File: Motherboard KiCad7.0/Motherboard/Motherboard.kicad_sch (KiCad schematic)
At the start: 52 parts, among them J1 USB_B_Micro, J2 SWD_01x04_Pin, J3 2-1445057-2, Q1 AO3400A, Q2 NMOS, SW1 SW_STM_RESET, SW2 SW_STM_BOOT_MODE, U1 STM32F103CBT6, U2 AMS1117-3.3, U3 LM66100DCKR, U4 LM66100DCKR, U5 LM66100DCKR, Y1 X322516MMB4SI

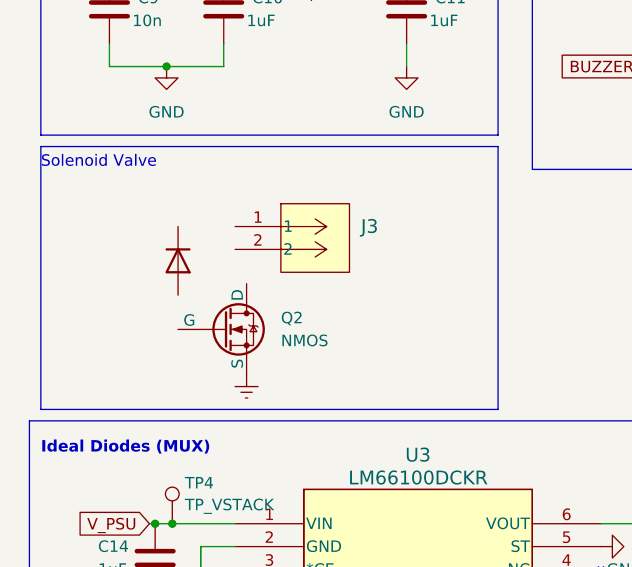
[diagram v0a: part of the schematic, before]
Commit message: Solenoid valve
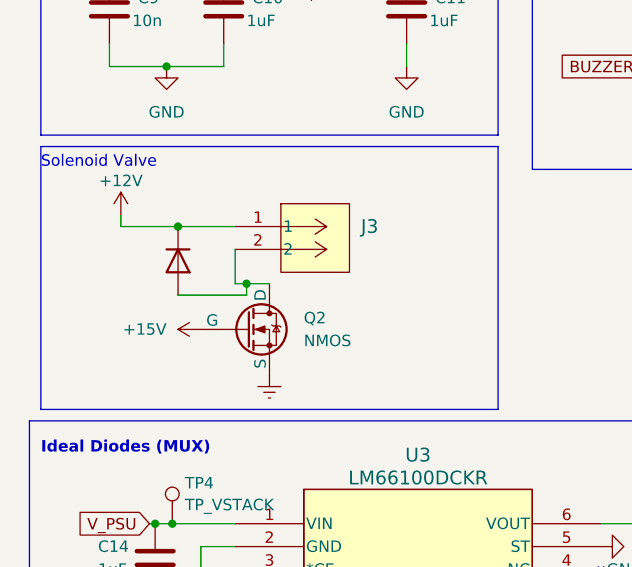
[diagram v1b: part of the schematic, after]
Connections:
- net +12V: now reaches J3.1
- net +12V: now also D6.1 (K)
- net at J3.2: now also D6.2 (A), Q2.1 (D)
- net +15V: now reaches Q2.2 (G)
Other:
- moved on the sheet: Q2
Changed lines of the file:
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@@
   (junction (at 175.26 110.49) (diameter 0) (color 0 0 0 0)
+  )
+  (junction (at 39.37 114.3) (diameter 0) (color 0 0 0 0)
+  )
+  (junction (at 31.75 107.95) (diameter 0) (color 0 0 0 0)
   )
   (junction (at 29.21 186.69) (diameter 0) (color 0 0 0 0)
@@
     (stroke (width 0) (type default))
   )
+  (wire (pts (xy 25.4 106.68) (xy 25.4 107.95))
+    (stroke (width 0) (type default))
+  )
   (wire (pts (xy 116.84 175.26) (xy 119.38 175.26))
     (stroke (width 0) (type default))
@@
     (stroke (width 0) (type default))
   )
+  (wire (pts (xy 39.37 114.3) (xy 41.91 114.3))
+    (stroke (width 0) (type default))
+  )
   (wire (pts (xy 241.935 67.31) (xy 245.11 67.31))
     (stroke (width 0) (type default))
@@
     (stroke (width 0) (type default))
   )
+  (wire (pts (xy 39.37 115.57) (xy 39.37 114.3))
+    (stroke (width 0) (type default))
+  )
   (wire (pts (xy 38.1 181.61) (xy 34.29 181.61))
     (stroke (width 0) (type default))
@@
     (stroke (width 0) (type default))
   )
+  (wire (pts (xy 38.1 107.95) (xy 31.75 107.95))
+    (stroke (width 0) (type default))
+  )
   (wire (pts (xy 101.6 36.83) (xy 111.76 36.83))
     (stroke (width 0) (type default))
@@
     (stroke (width 0) (type default))
   )
+  (wire (pts (xy 31.75 115.57) (xy 39.37 115.57))
+    (stroke (width 0) (type default))
+  )
   (wire (pts (xy 57.15 87.63) (xy 57.15 90.17))
     (stroke (width 0) (type default))
@@
     (stroke (width 0) (type default))
   )
+  (wire (pts (xy 38.1 114.3) (xy 39.37 114.3))
+    (stroke (width 0) (type default))
+  )
   (wire (pts (xy 260.35 88.9) (xy 264.16 88.9))
     (stroke (width 0) (type default))
@@
     (stroke (width 0) (type default))
   )
+  (wire (pts (xy 38.1 110.49) (xy 38.1 114.3))
+    (stroke (width 0) (type default))
+  )
   (wire (pts (xy 91.44 90.17) (xy 91.44 91.44))
     (stroke (width 0) (type default))
@@
   )
   (wire (pts (xy 175.26 29.21) (xy 172.72 29.21))
+    (stroke (width 0) (type default))
+  )
+  (wire (pts (xy 31.75 107.95) (xy 25.4 107.95))
     (stroke (width 0) (type default))
   )
@@
     )
   )
-  (symbol (lib_id "power:Earth") (at 39.37 124.46 0) (unit 1)
-    (in_bom yes) (on_board yes) (dnp no) (fields_autoplaced)
-    (property "Reference" "#PWR033" (at 39.37 130.81 0)
-      (effects (font (size 1.27 1.27)) hide)
-    )
-    (property "Value" "Earth" (at 39.37 128.27 0)
-      (effects (font (size 1.27 1.27)) hide)
-    )
-    (property "Footprint" "" (at 39.37 124.46 0)
-      (effects (font (size 1.27 1.27)) hide)
-    )
-    (property "Datasheet" "~" (at 39.37 124.46 0)
+  (symbol (lib_id "power:Earth") (at 41.91 124.46 0) (unit 1)
+    (in_bom yes) (on_board yes) (dnp no) (fields_autoplaced)
+    (property "Reference" "#PWR033" (at 41.91 130.81 0)
+      (effects (font (size 1.27 1.27)) hide)
+    )
+    (property "Value" "Earth" (at 41.91 128.27 0)
+      (effects (font (size 1.27 1.27)) hide)
+    )
+    (property "Footprint" "" (at 41.91 124.46 0)
+      (effects (font (size 1.27 1.27)) hide)
+    )
+    (property "Datasheet" "~" (at 41.91 124.46 0)
       (effects (font (size 1.27 1.27)) hide)
     )
@@
     )
   )
+  (symbol (lib_id "power:+12V") (at 25.4 106.68 0) (unit 1)
+    (in_bom yes) (on_board yes) (dnp no)
+    (property "Reference" "#PWR034" (at 25.4 110.49 0)
+      (effects (font (size 1.27 1.27)) hide)
+    )
+    (property "Value" "+12V" (at 25.4 102.87 0)
+      (effects (font (size 1.27 1.27)))
+    )
+    (property "Footprint" "" (at 25.4 106.68 0)
+      (effects (font (size 1.27 1.27)) hide)
+    )
+    (property "Datasheet" "" (at 25.4 106.68 0)
+      (effects (font (size 1.27 1.27)) hide)
+    )
+    (pin "1")
+    (instances
+      (project "Motherboard"
+        (path "/6c6aab7b-9fc7-4161-8073-41667e18c629"
+          (reference "#PWR034") (unit 1)
+        )
+      )
+    )
+  )
   (symbol (lib_id "Device:R") (at 228.6 134.62 180) (unit 1)
     (in_bom yes) (on_board yes) (dnp no) (fields_autoplaced)
@@
     )
   )
+  (symbol (lib_id "power:+15V") (at 34.29 119.38 90) (unit 1)
+    (in_bom yes) (on_board yes) (dnp no) (fields_autoplaced)
+    (property "Reference" "#PWR035" (at 38.1 119.38 0)
+      (effects (font (size 1.27 1.27)) hide)
+    )
+    (property "Value" "+15V" (at 30.48 119.38 90)
+      (effects (font (size 1.27 1.27)) (justify left))
+    )
+    (property "Footprint" "" (at 34.29 119.38 0)
+      (effects (font (size 1.27 1.27)) hide)
+    )
+    (property "Datasheet" "" (at 34.29 119.38 0)
+      (effects (font (size 1.27 1.27)) hide)
+    )
+    (pin "1")
+    (instances
+      (project "Motherboard"
+        (path "/6c6aab7b-9fc7-4161-8073-41667e18c629"
+          (reference "#PWR035") (unit 1)
+        )
+      )
+    )
+  )
   (symbol (lib_id "Device:R") (at 127 179.07 0) (unit 1)
     (in_bom yes) (on_board yes) (dnp no) (fields_autoplaced)
@@
     )
   )
-  (symbol (lib_id "Simulation_SPICE:NMOS") (at 36.83 119.38 0) (unit 1)
-    (in_bom yes) (on_board yes) (dnp no) (fields_autoplaced)
-    (property "Reference" "Q2" (at 43.18 118.11 0)
-      (effects (font (size 1.27 1.27)) (justify left))
-    )
-    (property "Value" "NMOS" (at 43.18 120.65 0)
-      (effects (font (size 1.27 1.27)) (justify left))
-    )
-    (property "Footprint" "" (at 41.91 116.84 0)
-      (effects (font (size 1.27 1.27)) hide)
-    )
-    (property "Datasheet" "https://ngspice.sourceforge.io/docs/ngspice-manual.pdf" (at 36.83 132.08 0)
-      (effects (font (size 1.27 1.27)) hide)
-    )
-    (property "Sim.Device" "NMOS" (at 36.83 136.525 0)
-      (effects (font (size 1.27 1.27)) hide)
-    )
-    (property "Sim.Type" "VDMOS" (at 36.83 138.43 0)
-      (effects (font (size 1.27 1.27)) hide)
-    )
-    (property "Sim.Pins" "1=D 2=G 3=S" (at 36.83 134.62 0)
-      (effects (font (size 1.27 1.27)) hide)
-    )
+  (symbol (lib_id "Simulation_SPICE:NMOS") (at 39.37 119.38 0) (unit 1)
+    (in_bom yes) (on_board yes) (dnp no) (fields_autoplaced)
+    (property "Reference" "Q2" (at 45.72 118.11 0)
+      (effects (font (size 1.27 1.27)) (justify left))
+    )
+    (property "Value" "NMOS" (at 45.72 120.65 0)
+      (effects (font (size 1.27 1.27)) (justify left))
+    )
+    (property "Footprint" "" (at 44.45 116.84 0)
+      (effects (font (size 1.27 1.27)) hide)
+    )
+    (property "Datasheet" "https://ngspice.sourceforge.io/docs/ngspice-manual.pdf" (at 39.37 132.08 0)
+      (effects (font (size 1.27 1.27)) hide)
+    )
+    (property "Sim.Device" "NMOS" (at 39.37 136.525 0)
+      (effects (font (size 1.27 1.27)) hide)
+    )
+    (property "Sim.Type" "VDMOS" (at 39.37 138.43 0)
+      (effects (font (size 1.27 1.27)) hide)
+    )
+    (property "Sim.Pins" "1=D 2=G 3=S" (at 39.37 134.62 0)
+      (effects (font (size 1.27 1.27)) hide)
+    )
